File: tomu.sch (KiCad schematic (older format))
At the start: 15 parts, among them P1 USART0, P2 DEBUG, P3 USB-PCB, U1 MKL27Z256VFM4

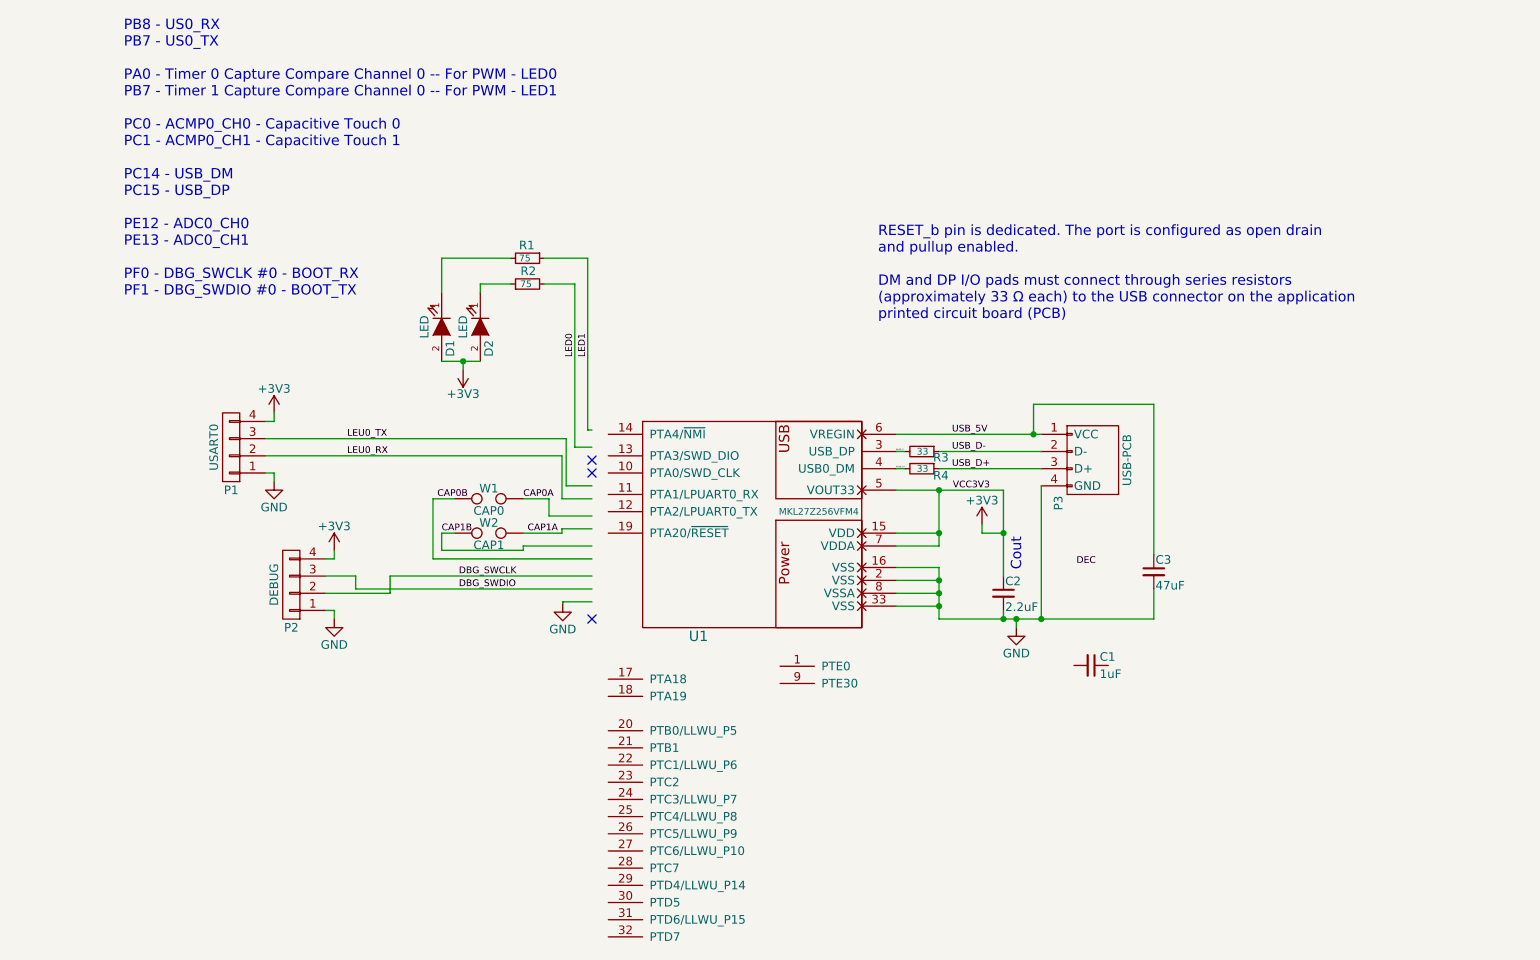
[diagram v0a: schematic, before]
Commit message: Lots of small updates.
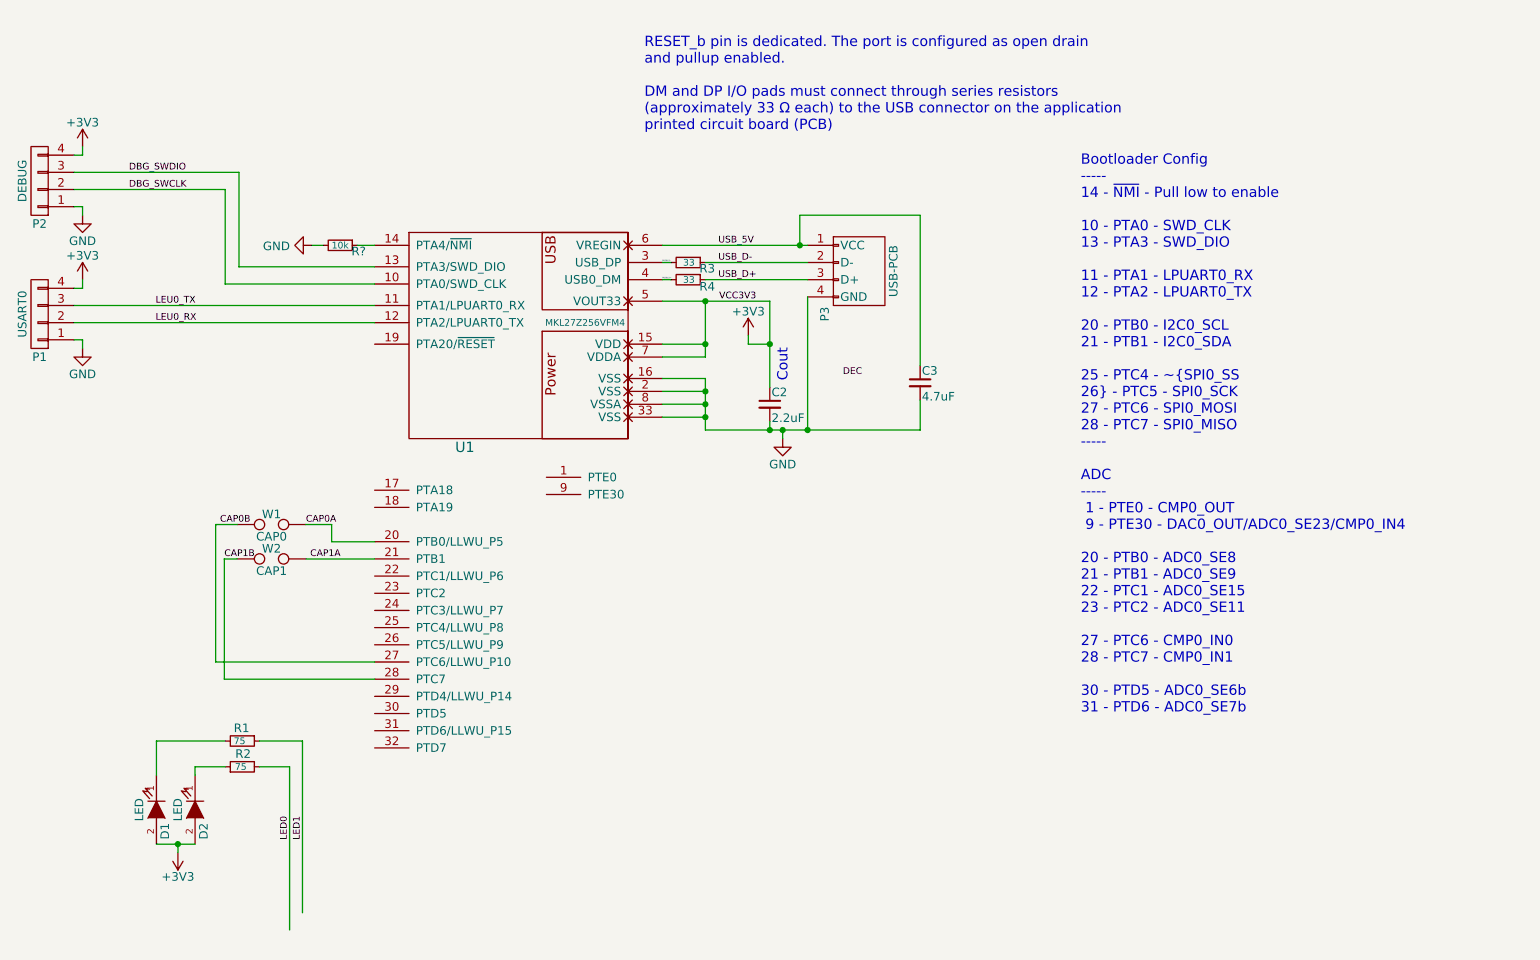
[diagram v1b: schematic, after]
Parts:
- removed C1: 1uF, Capacitors_SMD:C_0402, symbol C_Small
- added R?: 10k, Resistors_SMD:R_0402, symbol R_Small
- C3: value 47uF -> 4.7uF
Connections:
- wire segments 73 -> 63
- no-connect marks 3 -> 0
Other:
- note added: "Bootloader Config\n-----\n14 - ~NMI~ - Pull low to enable\n\n10 - PTA0 - SWD_CLK\n13 - PTA3 - SWD_DIO\n\n11 - PTA1 - LPUART0_RX\n12 - PTA2 - LPUART0_TX\n\n20 - PTB0 - I2C0_SCL\n21 - PTB1 - I2C0_SDA\n\n25 - PTC4 - ~SPI0_SS\n26 - PTC5 - SPI0_SCK\n27 - PTC6 - SPI0_MOSI\n28 - PTC7 - SPI0_MISO\n-----\n\nADC \n-----\n 1 - PTE0 - CMP0_OUT\n 9 - PTE30 - DAC0_OUT/ADC0_SE23/CMP0_IN4\n\n20 - PTB0 - ADC0_SE8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"
- note removed: "PB8 - US0_RX\nPB7 - US0_TX\n\nPA0 - Timer 0 Capture Compare Channel 0 -- For PWM - LED0 \nPB7 - Timer 1 Capture Compare Channel 0 -- For PWM - LED1\n\nPC0 - ACMP0_CH0 - Capacitive Touch 0\nPC1 - ACMP0_CH1 - Capacitive Touch 1\n\nPC14 - USB_DM\nPC15 - USB_DP\n\nPE12 - ADC0_CH0\nPE13 - ADC0_CH1\n\nPF0 - DBG_SWCLK #0 - BOOT_RX\nPF1 - DBG_SWDIO #0 - BOOT_TX\n\n"
- moved on the sheet: C2, C3, D1, D2, P1, P2, P3, R1, R2, R3, R4, U1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
